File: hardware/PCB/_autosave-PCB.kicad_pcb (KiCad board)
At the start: 2 copper layers, 30.4 x 52.6 mm, 42 parts, among them J1 Conn_01x02_Pin, J2 USB_C_Receptacle_USB2.0_14P, J3 Conn_01x04_Pin, Q1 BC807, Q2 BC817, Q3 BC817, SW1 SW_Push, SW2 SW_Push, U1 ESP32-C6-MINI-1, U2 AP3015, U3 MCP1700x-330xxTT

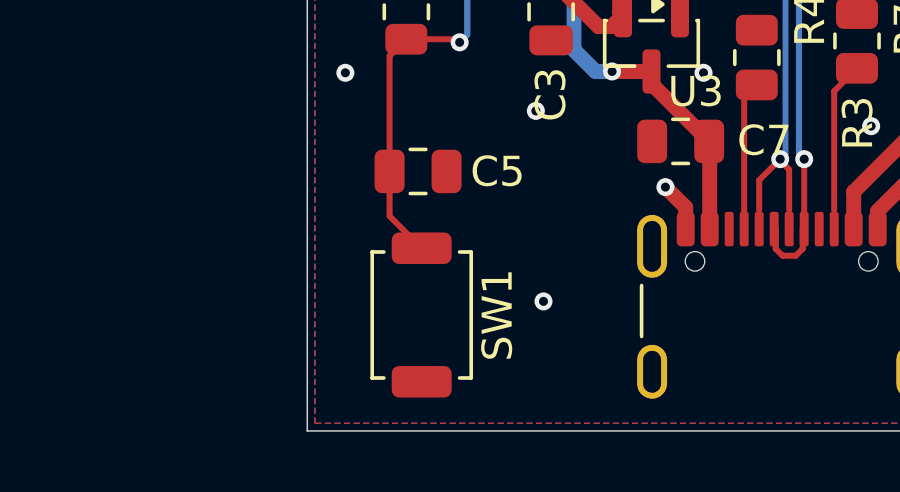
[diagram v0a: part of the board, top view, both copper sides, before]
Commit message: WIP
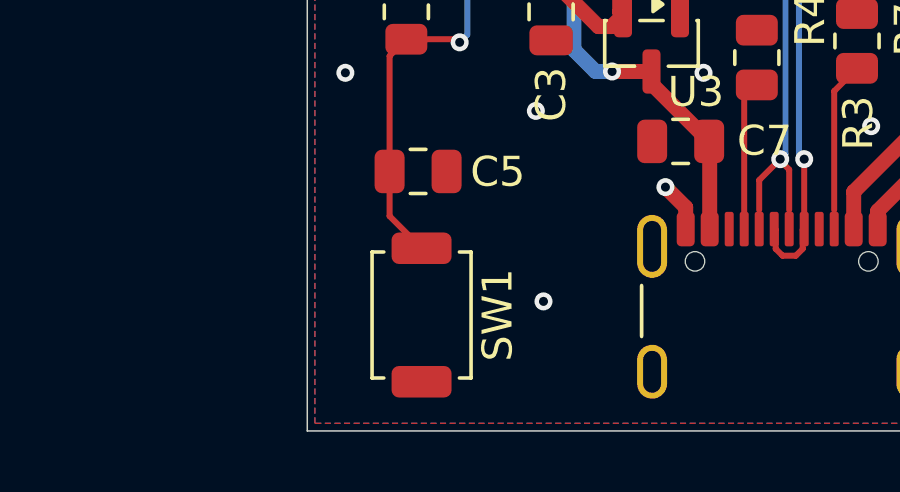
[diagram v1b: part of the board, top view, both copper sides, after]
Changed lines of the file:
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@@
 	(footprint "Button_Switch_SMD:SW_SPST_TS-1088-xR025"
 		(layer "F.Cu")
-		(at 134.37 86.305 90)
+		(at 134.366 86.305 90)
 		(descr "SMD Tactile Switch, 3.9x3x2.5 mm, https://lcsc.com/datasheet/lcsc_datasheet_2504101957_XUNPU-TS-1088-AR02016_C720477.pdf")
 		(tags "Tactile Switch")
@@
 	)
 	(segment
-		(start 141.224 47.8555)
-		(end 143.51 47.8555)
+		(start 147.2655 47.8555)
+		(end 147.574 47.547)
 		(width 0.5)
 		(layer "F.Cu")
@@
 	)
 	(segment
-		(start 142.966 42.1965)
-		(end 142.966 47.3115)
+		(start 141.224 47.8555)
+		(end 143.51 47.8555)
 		(width 0.5)
 		(layer "F.Cu")
@@
 	)
 	(segment
-		(start 147.2655 47.8555)
-		(end 147.574 47.547)
+		(start 142.966 42.1965)
+		(end 142.966 47.3115)
 		(width 0.5)
 		(layer "F.Cu")
